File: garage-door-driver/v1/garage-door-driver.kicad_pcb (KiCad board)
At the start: 2 copper layers, 45 x 45 mm, 5 parts, among them J1 Screw_Terminal_01x04

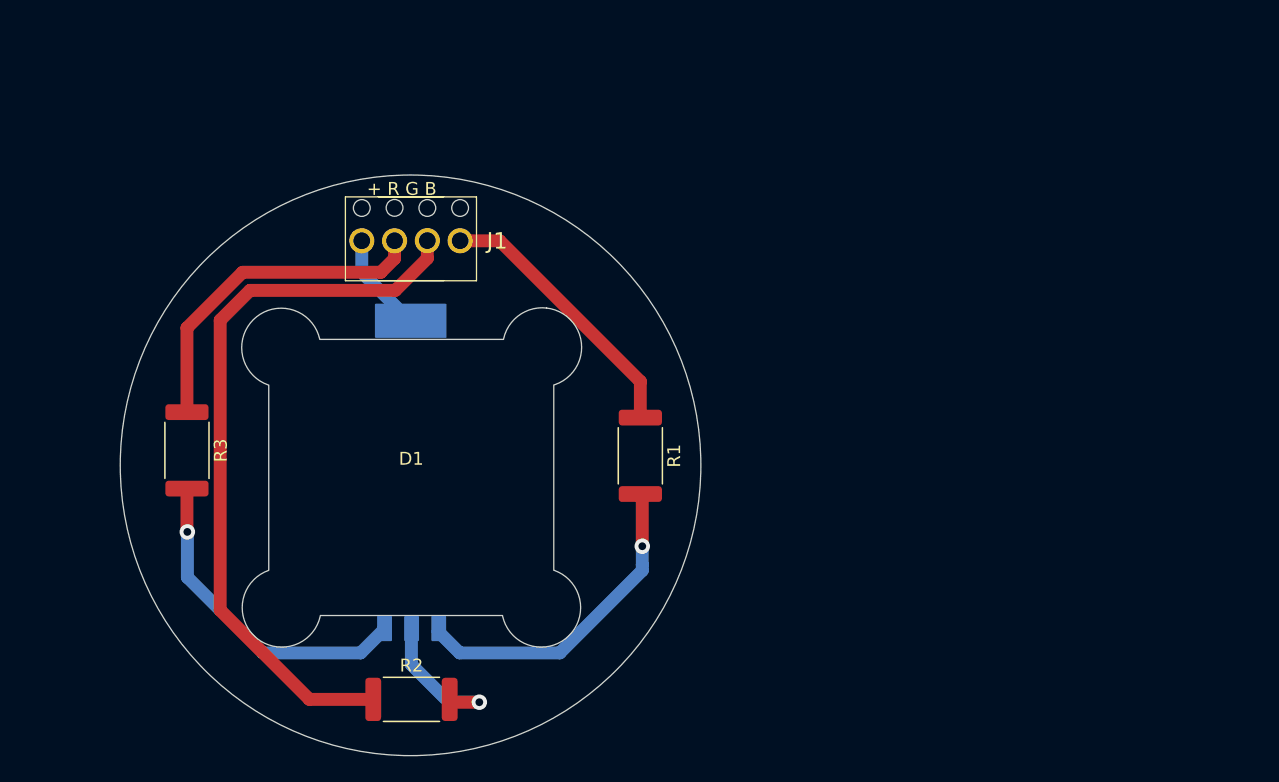
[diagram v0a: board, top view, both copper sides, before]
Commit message: clean PCB + add edge cuts
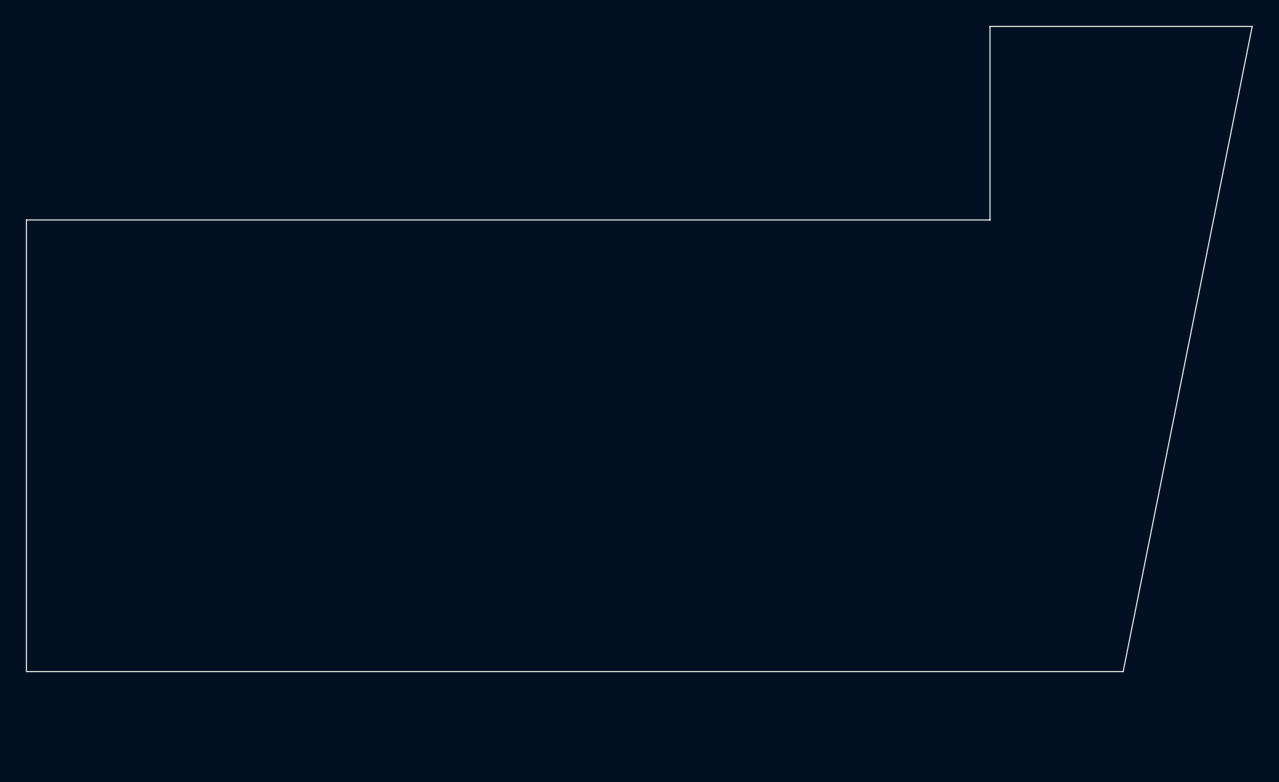
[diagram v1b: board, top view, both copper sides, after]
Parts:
- removed D1: LED_ARGB, mylife-footprints:LED RGB 10W
- removed J1: Screw_Terminal_01x04, mylife-footprints:RS PRO Terminal Small x4
- removed R1, R2: 5.1Ω/1W, Resistor_SMD:R_2512_6332Metric
- removed R3: 10Ω/1W, Resistor_SMD:R_2512_6332Metric
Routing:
- net Net-(J1-Pin_2): track 56.6 -> 0.00 mm
- net Net-(J1-Pin_3): track 26.2 -> 0.00 mm
- net Net-(D1-RK): track 25.3 -> 0.00 mm, vias 1 -> 0
- net Net-(D1-BK): track 25.2 -> 0.00 mm, vias 1 -> 0
- net Net-(J1-Pin_1): track 21.3 -> 0.00 mm
- net Net-(D1-GK): track 11.6 -> 0.00 mm, vias 1 -> 0
- net Net-(D1-A): track 7.84 -> 0.00 mm
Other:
- board size 45 x 45 mm -> 95 x 50 mm
- board text removed: "+ R G B"
